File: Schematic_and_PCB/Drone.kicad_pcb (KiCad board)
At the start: 2 copper layers, 218.4 x 101.6 mm, 0 parts

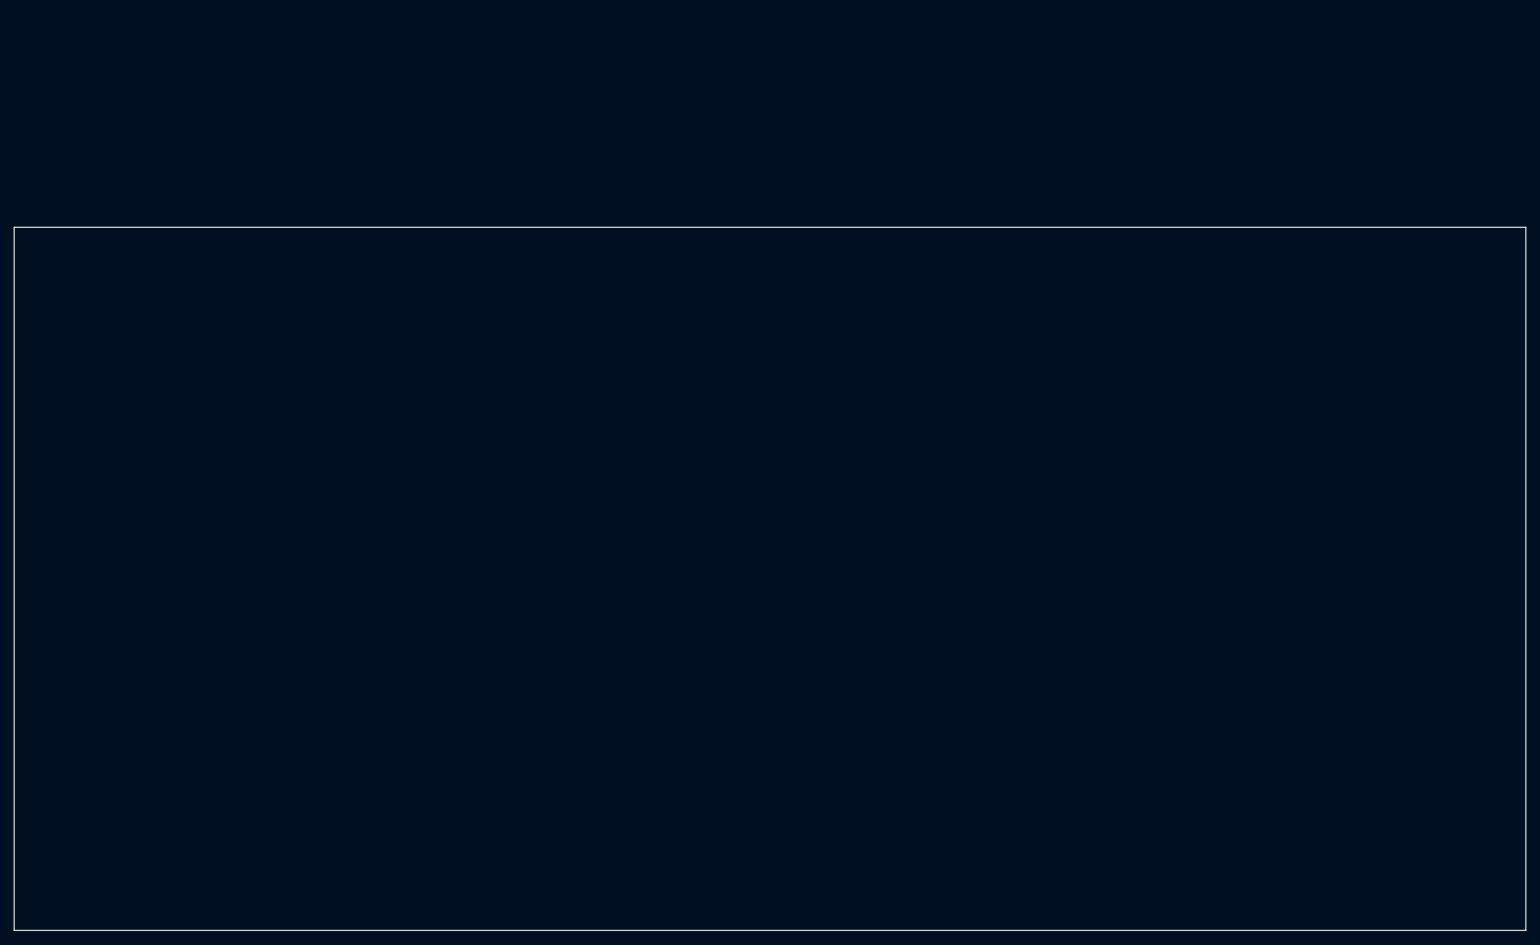
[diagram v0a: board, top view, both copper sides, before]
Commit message: Schematic and PCB design
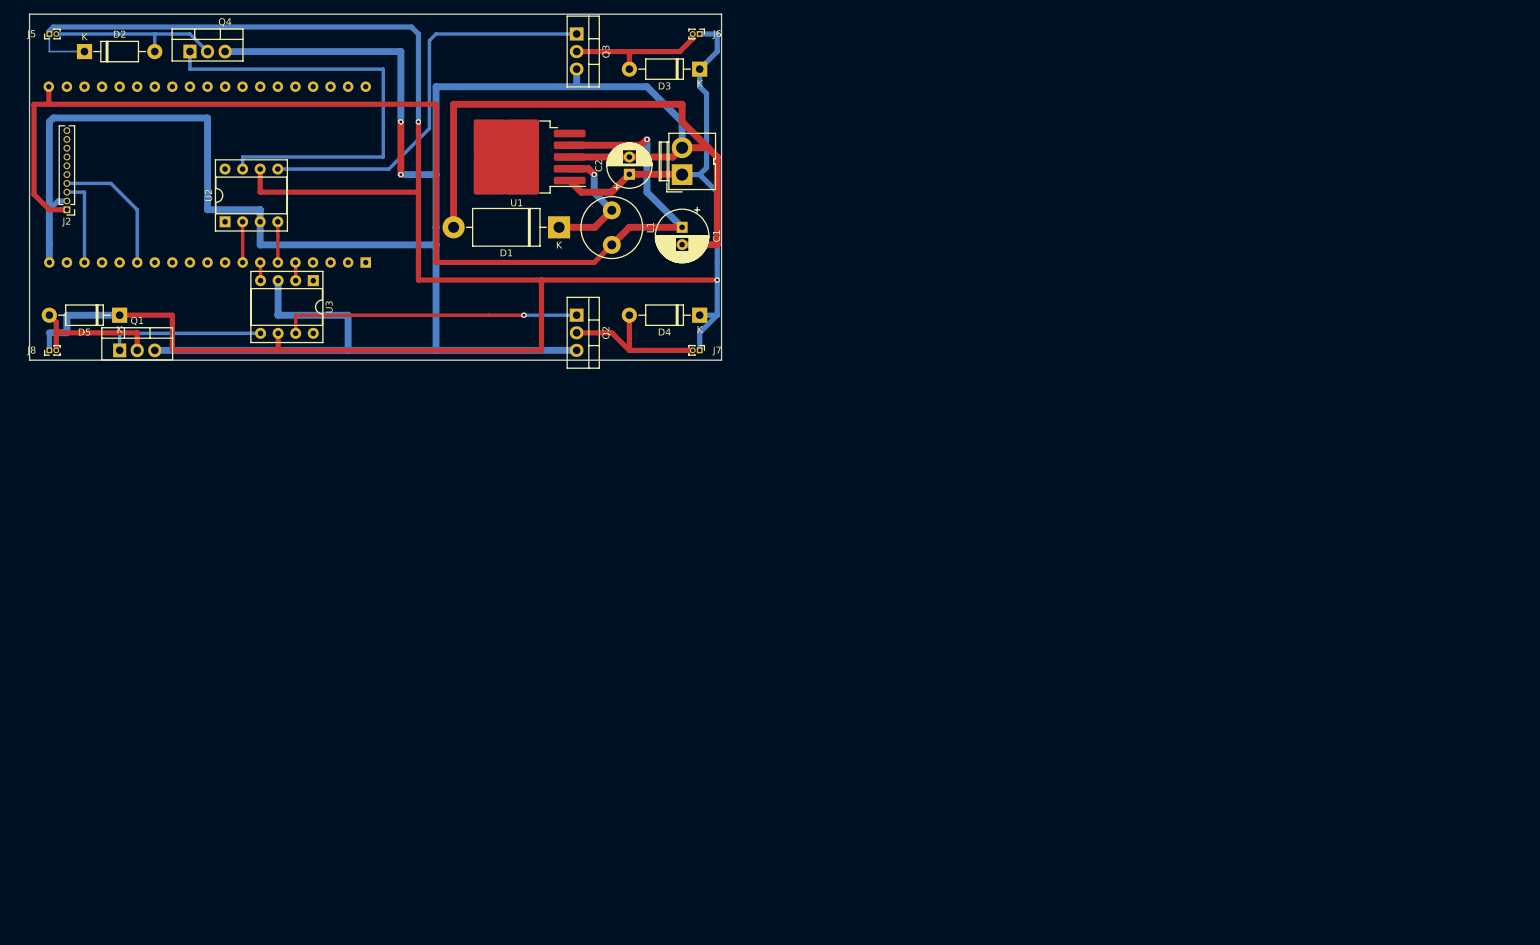
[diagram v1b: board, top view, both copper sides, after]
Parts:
- added C1: 1000uF, Capacitor_THT:CP_Radial_D7.5mm_P2.50mm, F.Cu at (114.3, 50.8)
- added C2: 100uF, Capacitor_THT:CP_Radial_D6.3mm_P2.50mm, F.Cu at (106.7, 43.1)
- added D1: 1N5822, Diode_THT:D_DO-201AD_P15.24mm_Horizontal, F.Cu at (96.5, 50.8)
- added D2: 1N5817, Diode_THT:D_DO-41_SOD81_P10.16mm_Horizontal, F.Cu at (27.9, 25.4)
- added D3: 1N5817, Diode_THT:D_DO-41_SOD81_P10.16mm_Horizontal, F.Cu at (116.8, 27.9)
- added D4: 1N5817, Diode_THT:D_DO-41_SOD81_P10.16mm_Horizontal, F.Cu at (116.8, 63.5)
- added D5: 1N5817, Diode_THT:D_DO-41_SOD81_P10.16mm_Horizontal, F.Cu at (33.0, 63.5)
- added ESP32: NodeMCU_DevKitC_v4, Module:NodeMCU DevKitC v4, B.Cu at (68.6, 55.9)
- added J1: BATT, Connector:JWT_A3963_1x02_P3.96mm_Vertical, F.Cu at (114.3, 43.2)
- added J2: PinHeader_1x10_P1.27mm_Vertical, Connector_PinHeader_1.27mm:PinHeader_1x10_P1.27mm_Vertical, F.Cu at (25.4, 48.3)
- added J5: Motor 4, Connector_PinHeader_1.00mm:PinHeader_1x02_P1.00mm_Vertical, F.Cu at (22.9, 22.9)
- added J6: Motor 1, Connector_PinHeader_1.00mm:PinHeader_1x02_P1.00mm_Vertical, F.Cu at (116.8, 22.9)
- added J7: Motor 2, Connector_PinHeader_1.00mm:PinHeader_1x02_P1.00mm_Vertical, F.Cu at (116.8, 68.6)
- added J8: Motor 3, Connector_PinHeader_1.00mm:PinHeader_1x02_P1.00mm_Vertical, F.Cu at (22.9, 68.6)
- added L1: 100uH 1A, Inductor_THT:L_Radial_D8.7mm_P5.00mm_Fastron_07HCP, F.Cu at (104.1, 48.3)
- added Q1: IRLZ34N, Package_TO_SOT_THT:TO-220-3_Vertical, F.Cu at (33.0, 68.6)
- added Q2: IRLZ34N, Package_TO_SOT_THT:TO-220-3_Vertical, F.Cu at (99.1, 63.5)
- added Q3: IRLZ34N, Package_TO_SOT_THT:TO-220-3_Vertical, F.Cu at (99.1, 22.9)
- added Q4: IRLZ34N, Package_TO_SOT_THT:TO-220-3_Vertical, F.Cu at (43.2, 25.4)
- added U1: LM2576HVS-3.3, Package_TO_SOT_SMD:TO-263-5_TabPin3, F.Cu at (90.4, 40.6)
- added U2: TC4424EPA, Package_DIP:DIP-8_W7.62mm_Socket, F.Cu at (48.2, 50.0)
- added U3: TC4424EPA, Package_DIP:DIP-8_W7.62mm_Socket, F.Cu at (61.0, 58.5)
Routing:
- net GND: track 0.00 -> 408.2 mm, vias 0 -> 2
- net Net-(D2-K): track 0.00 -> 334.9 mm, vias 0 -> 2
- net Net-(ESP32-Pin_1): track 0.00 -> 166.2 mm, vias 0 -> 1
- net Net-(Q4-G): track 0.00 -> 65.2 mm
- net Net-(Q3-G): track 0.00 -> 58.7 mm
- net (no net): track 0.00 -> 49.1 mm
- net Net-(Q2-G): track 0.00 -> 43.3 mm, vias 0 -> 1
- net Net-(D2-A): track 0.00 -> 25.5 mm
- net Net-(D4-A): track 0.00 -> 22.9 mm
- net Net-(Q1-G): track 0.00 -> 22.9 mm
- net Net-(D3-A): track 0.00 -> 20.8 mm
- net Net-(D5-A): track 0.00 -> 19.7 mm
- net Net-(D1-K): track 0.00 -> 18.7 mm, vias 0 -> 1
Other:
- board size 218.4 x 101.6 mm -> 100 x 50 mm
